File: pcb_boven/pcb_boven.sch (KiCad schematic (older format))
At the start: 38 parts, among them U1 miniIMU-9_v6, U2 openMV_M7_R2

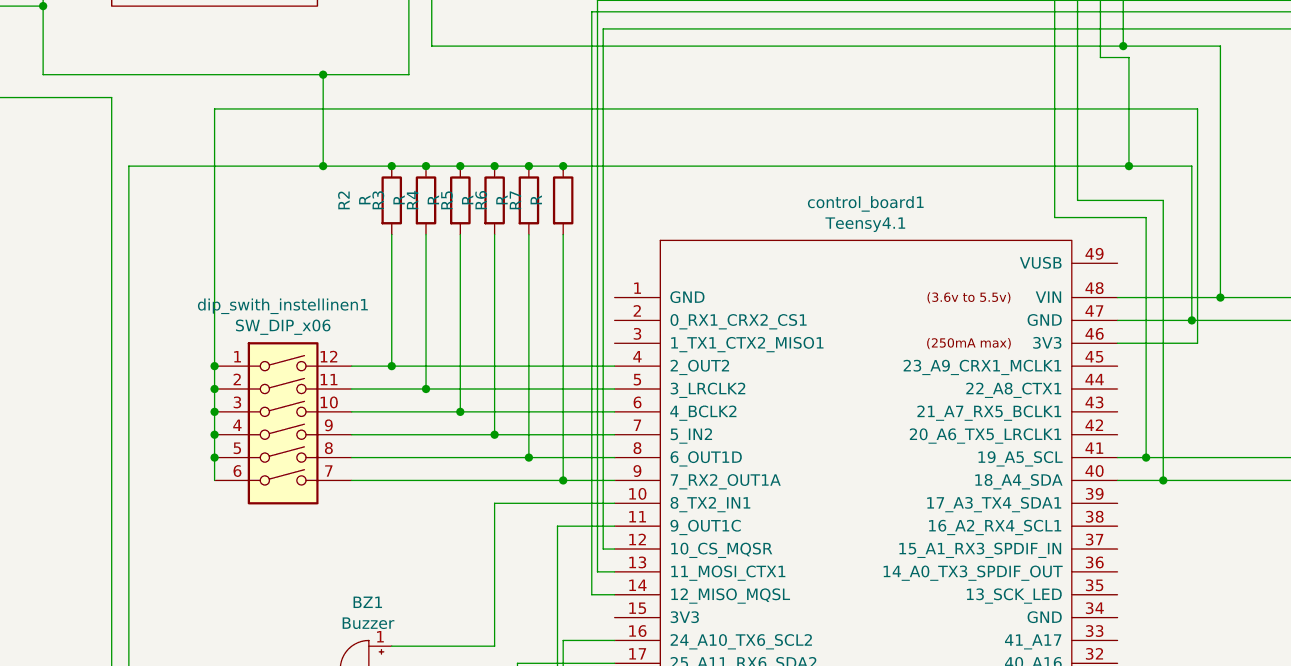
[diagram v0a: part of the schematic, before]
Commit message: 4dip
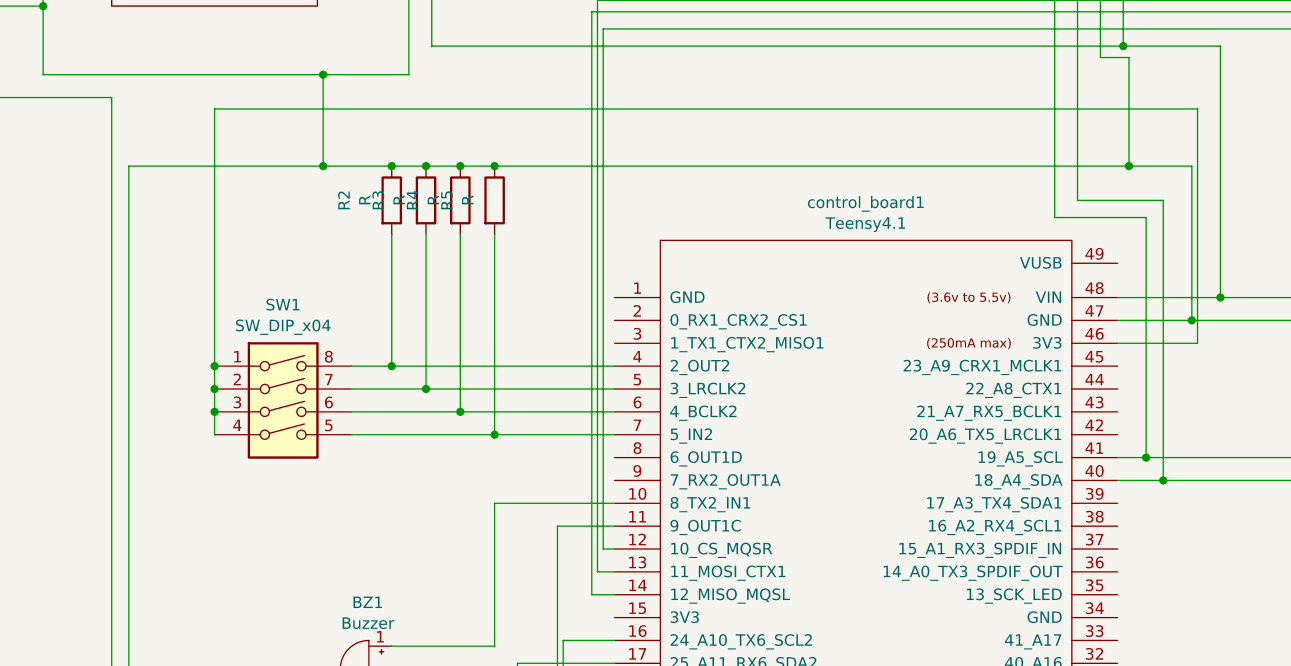
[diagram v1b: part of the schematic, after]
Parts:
- removed R6, R7: R, custom:resistor, symbol Device:R
- removed dip_swith_instellinen1: SW_DIP_x06, custom:dipswitch6, symbol Switch:SW_DIP_x06
- added SW1: SW_DIP_x04, custom:dipswitch4, symbol Switch:SW_DIP_x04
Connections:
- net at R2.2, control_board1.4 (2_OUT2): now also SW1.8
- net at control_board1.46 (3V3): now also SW1.1, SW1.2, SW1.3, SW1.4
- net at R3.2, control_board1.5 (3_LRCLK2): now also SW1.7
- net at R4.2, control_board1.6 (4_BCLK2): now also SW1.6
- net at R5.2, control_board1.7 (5_IN2): now also SW1.5
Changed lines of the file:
@@
-$EndComp
-$Comp
-L Switch:SW_DIP_x06 dip_swith_instellinen1
-U 1 1 66364D70
-P 3575 7200
-F 0 "dip_swith_instellinen1" H 3575 7767 50  0000 C CNN
-F 1 "SW_DIP_x06" H 3575 7676 50  0000 C CNN
-F 2 "custom:dipswitch6" H 3575 7200 50  0001 C CNN
-F 3 "~" H 3575 7200 50  0001 C CNN
-	1    3575 7200
-	1    0    0    -1
 $EndComp
 $Comp
@@
 $EndComp
 $Comp
-L Device:R R6
-U 1 1 66553C02
-P 4650 6175
-F 0 "R6" V 4443 6175 50  0000 C CNN
-F 1 "R" V 4534 6175 50  0000 C CNN
-F 2 "custom:resistor" V 4580 6175 50  0001 C CNN
-F 3 "~" H 4650 6175 50  0001 C CNN
-	1    4650 6175
-	1    0    0    -1
-$EndComp
-$Comp
-L Device:R R7
-U 1 1 6655A960
-P 4800 6175
-F 0 "R7" V 4593 6175 50  0000 C CNN
-F 1 "R" V 4684 6175 50  0000 C CNN
-F 2 "custom:resistor" V 4730 6175 50  0001 C CNN
-F 3 "~" H 4800 6175 50  0001 C CNN
-	1    4800 6175
-	1    0    0    -1
-$EndComp
-$Comp
 L Device:R R1
 U 1 1 665A1C89
@@
 	5025 7200 4500 7200
 Wire Wire Line
-	3875 7300 4650 7300
-Wire Wire Line
 	4050 6325 4050 6900
 Connection ~ 4050 6900
@@
 	4500 7200 3875 7200
 Wire Wire Line
-	4650 6325 4650 7300
-Connection ~ 4650 7300
-Wire Wire Line
-	4650 7300 5025 7300
-Wire Wire Line
-	4800 6325 4800 7400
-Wire Wire Line
-	3875 7400 4800 7400
-Connection ~ 4800 7400
-Wire Wire Line
-	4800 7400 5025 7400
-Wire Wire Line
-	3275 7400 3275 7300
-Wire Wire Line
-	3275 7300 3275 7200
-Connection ~ 3275 7300
-Wire Wire Line
 	3275 7200 3275 7100
-Connection ~ 3275 7200
 Wire Wire Line
 	3275 7000 3275 6900
@@
 Wire Wire Line
 	4350 6025 4500 6025
-Wire Wire Line
-	4650 6025 4800 6025
-Wire Wire Line
-	4650 6025 4500 6025
-Connection ~ 4650 6025
 Connection ~ 4500 6025
 Wire Wire Line
@@
 Connection ~ 4200 6025
 Wire Wire Line
-	4800 6025 7275 6025
-Wire Wire Line
 	7550 6025 7550 6700
-Connection ~ 4800 6025
 Connection ~ 7550 6700
 Wire Wire Line
@@
 Wire Wire Line
 	8825 7100 10325 7100
+$Comp
+L Switch:SW_DIP_x04 SW1
+U 1 1 666FC3F3
+P 3575 7100
+F 0 "SW1" H 3575 7567 50  0000 C CNN
+F 1 "SW_DIP_x04" H 3575 7476 50  0000 C CNN
+F 2 "custom:dipswitch4" H 3575 7100 50  0001 C CNN
+F 3 "~" H 3575 7100 50  0001 C CNN
+	1    3575 7100
+	1    0    0    -1
+$EndComp
+Wire Wire Line
+	4500 6025 7275 6025
 $EndSCHEMATC
